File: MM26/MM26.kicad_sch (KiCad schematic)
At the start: 18 parts, among them J1 B2B-PH-K-S, J2 B2B-PH-K-S, J3 Conn_01x06_Pin, J4 Conn_01x06_Pin, J5 Conn_01x03_Pin, J6 Conn_01x03_Pin, J7 Conn_01x03_Pin, J8 Conn_01x03_Pin, J9 Conn_01x03_Pin, SW1 CL-SB-12A-01T, U1 AZ1117IH-3.3TRG1, U2 NUCLEO-L476RG, U3 ISM330DHCX, U4 SSD1306, U5 L293DD

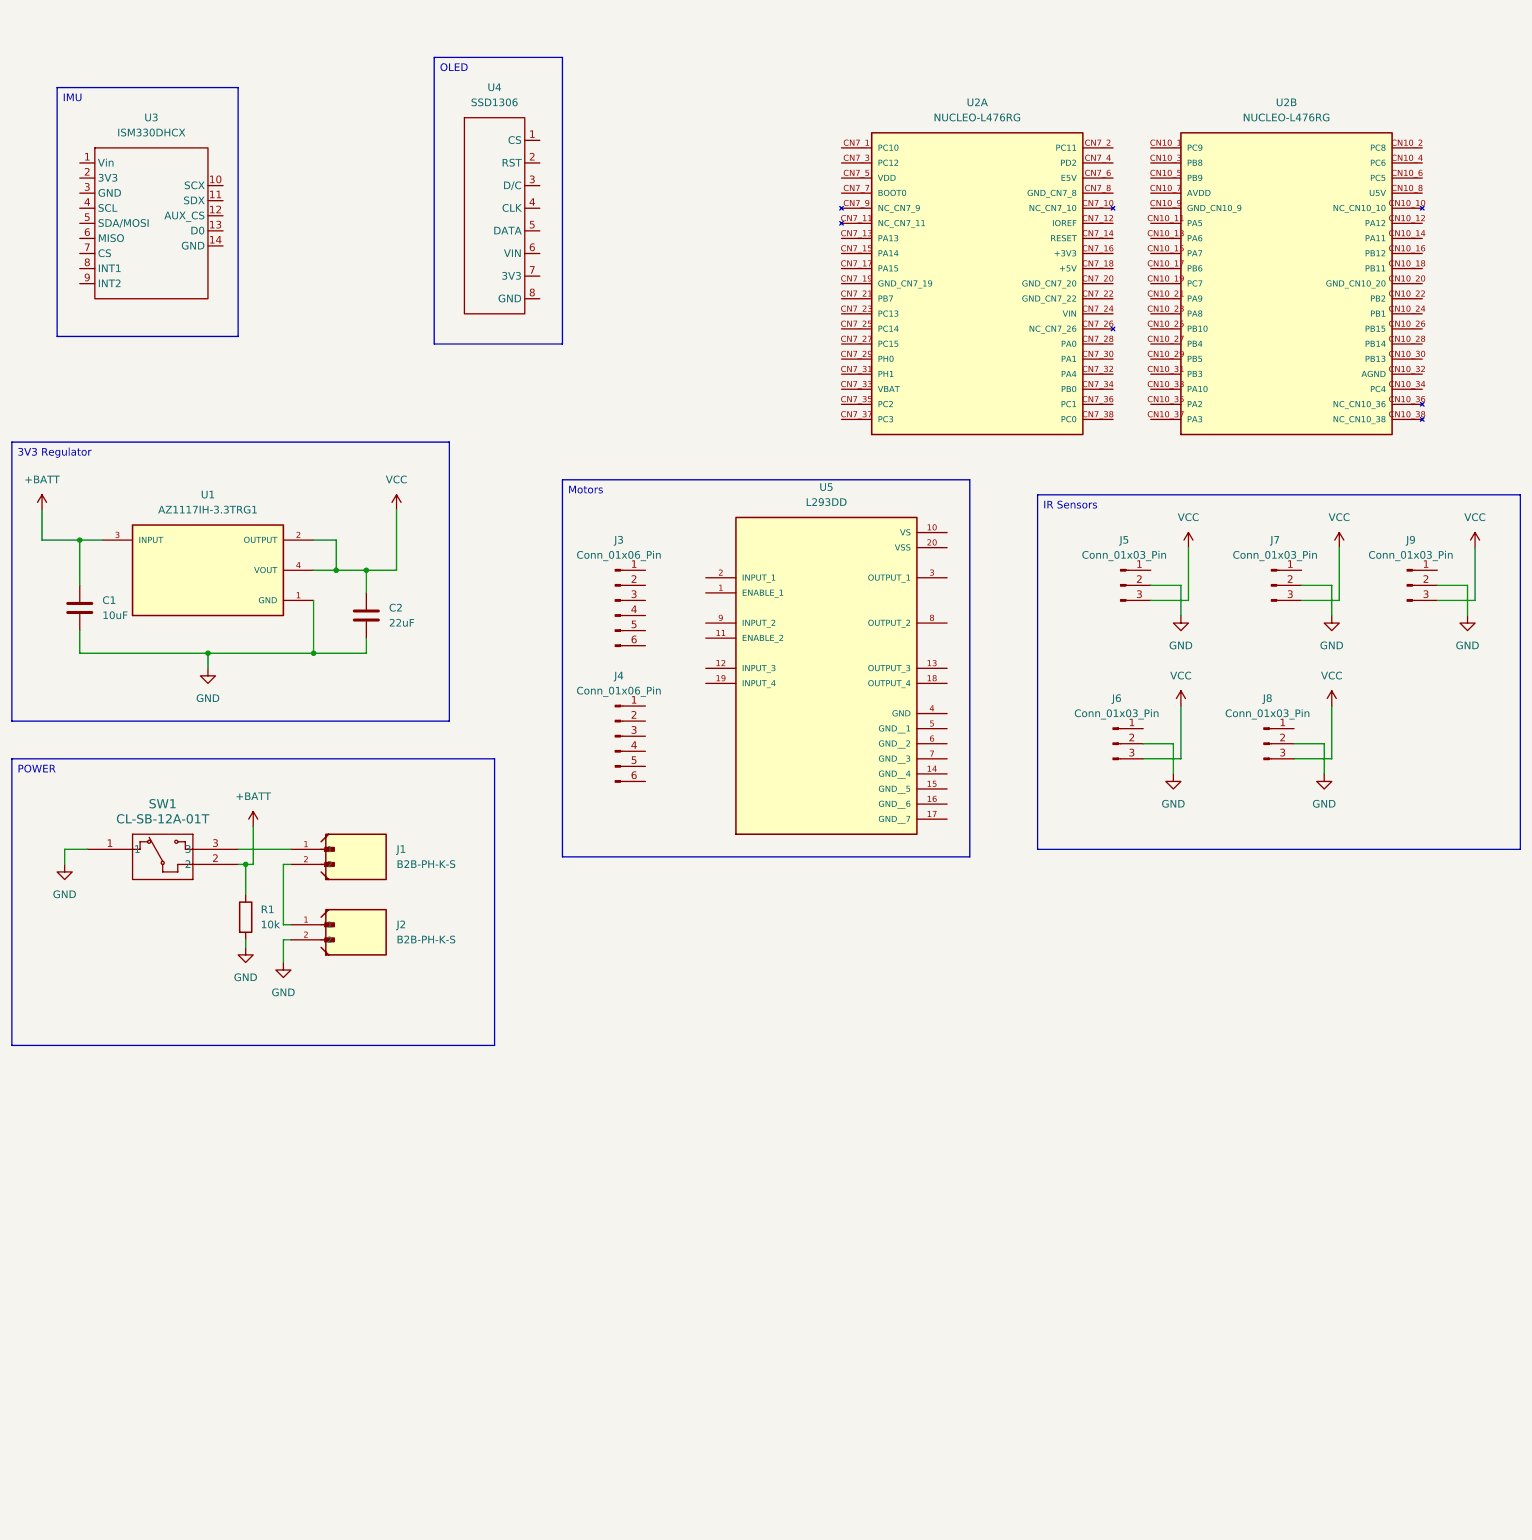
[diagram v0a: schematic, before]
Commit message: H Bridge Wiring
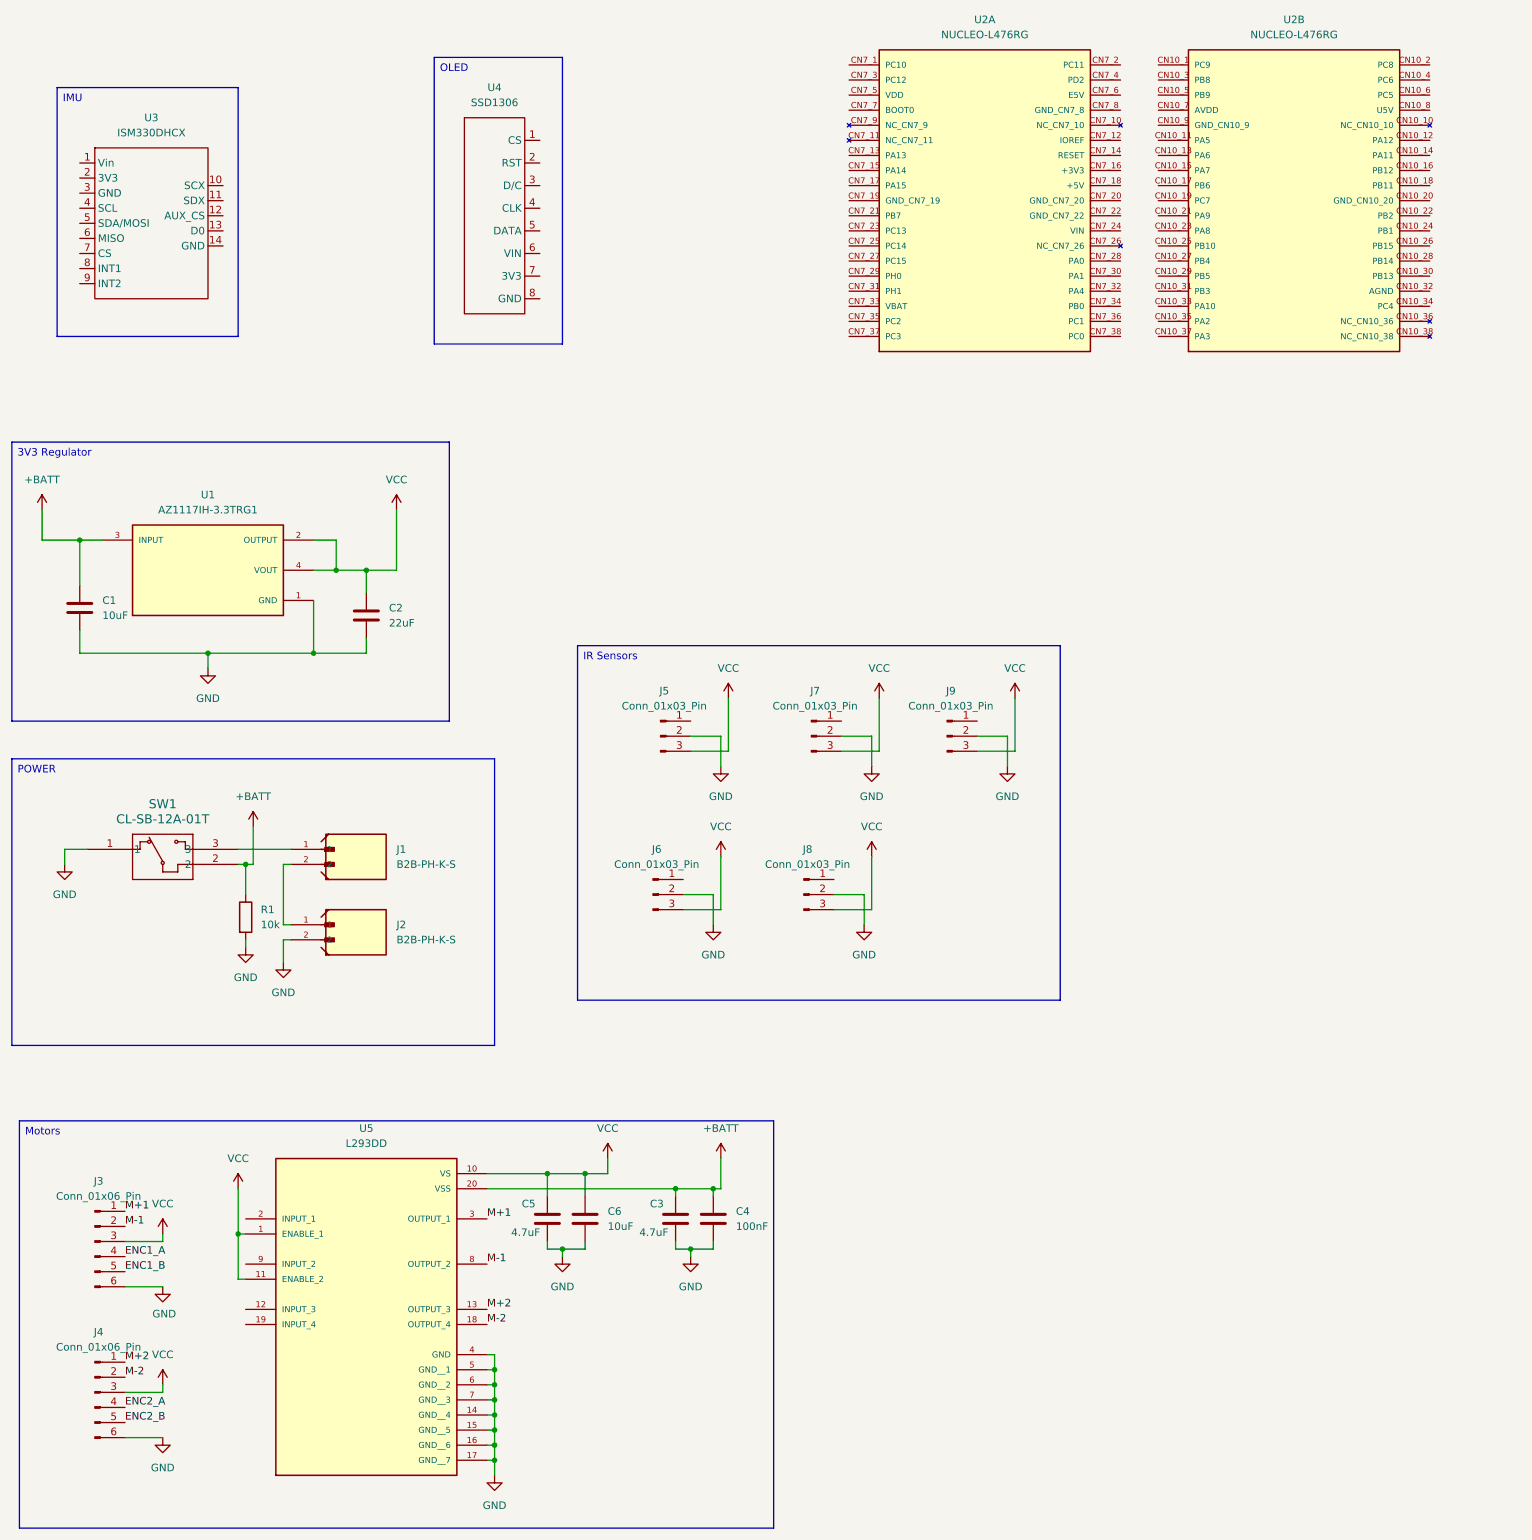
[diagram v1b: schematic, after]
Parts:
- added C3, C5: 4.7uF, symbol Device:C
- added C4: 100nF, symbol Device:C
- added C6: 10uF, symbol Device:C
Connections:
- net +BATT: now also U5.20 (VSS), C3.1, C4.1
- net GND: now also J3.6 (Pin_6), J4.6 (Pin_6), U5.14 (GND__4), U5.15 (GND__5), U5.16 (GND__6), U5.17 (GND__7), U5.4 (GND), U5.5 (GND__1), U5.6 (GND__2), U5.7 (GND__3), C3.2, C4.2, C5.2, C6.2
- net VCC: now also J3.3 (Pin_3), J4.3 (Pin_3), U5.1 (ENABLE_1), U5.10 (VS), U5.11 (ENABLE_2), C5.1, C6.1
- net M+2: now reaches J4.1 (Pin_1)
- net M+2: now also U5.13 (OUTPUT_3)
- net M-2: now reaches J4.2 (Pin_2)
- net M-2: now also U5.18 (OUTPUT_4)
- net ENC2_A: now reaches J4.4 (Pin_4)
- net ENC2_B: now reaches J4.5 (Pin_5)
- net M+1: now reaches U5.3 (OUTPUT_1)
- net M+1: now also J3.1 (Pin_1)
- net M-1: now reaches U5.8 (OUTPUT_2)
- net M-1: now also J3.2 (Pin_2)
- net ENC1_A: now reaches J3.4 (Pin_4)
- net ENC1_B: now reaches J3.5 (Pin_5)
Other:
- moved on the sheet: J3, J4, J5, J6, J7, J8, J9, U2A, U2B, U5
